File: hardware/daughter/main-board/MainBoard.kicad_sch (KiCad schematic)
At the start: 15 parts, among them J1 Conn_01x03_Pin, J2 Conn_01x03_Pin, J3 Conn_01x03_Pin, J4 Conn_01x03_Pin, SW1 SW_SP3T, SW2 SW_SP3T, U1 CD22M3494MQZ, U2 LM7321MAX/NOPB, U3 TL071, U4 TL071, U5 TL071, U6 TL071

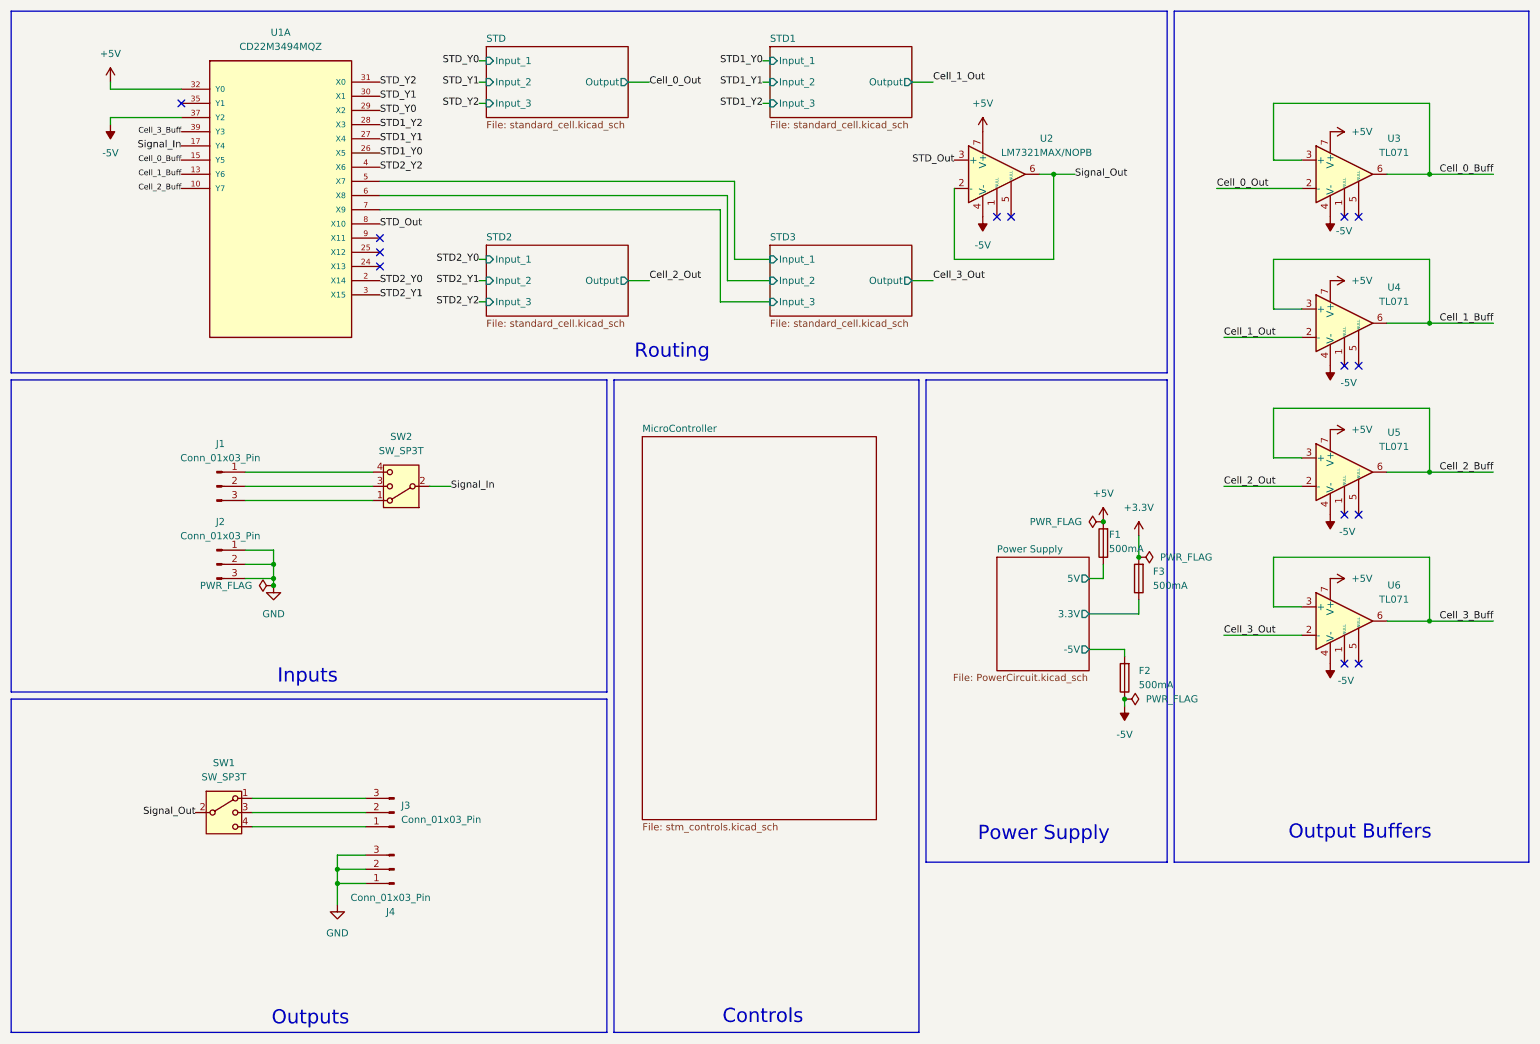
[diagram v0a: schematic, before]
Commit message: Updated daughter board schematic
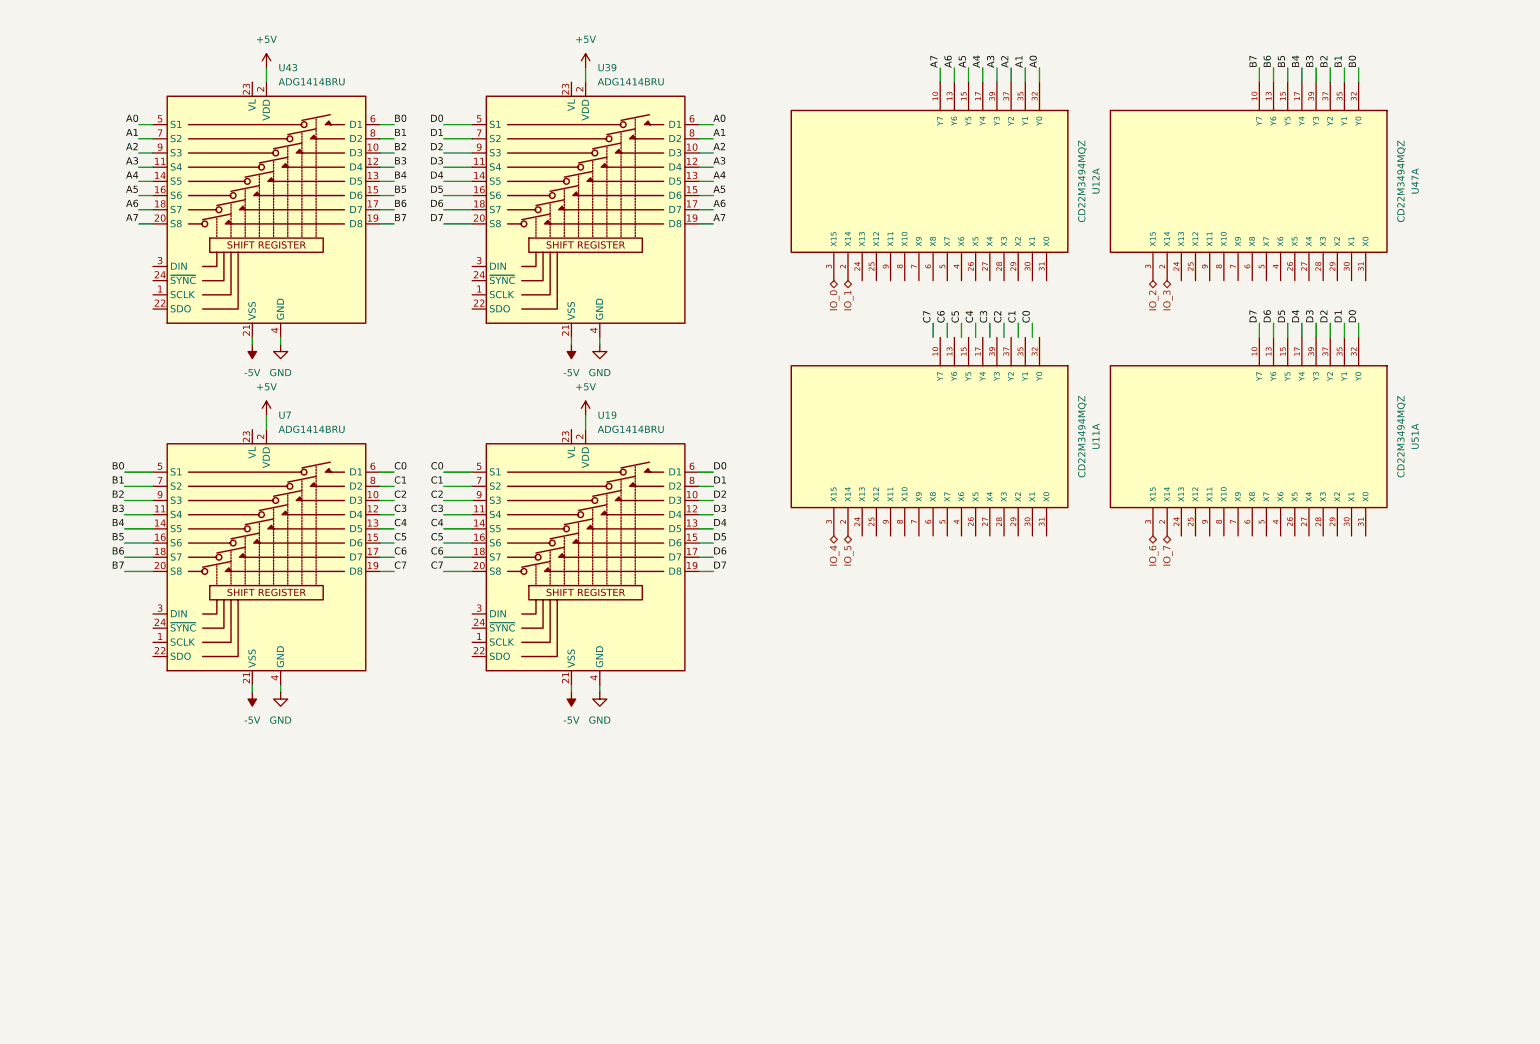
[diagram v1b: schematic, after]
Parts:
- removed F1, F2, F3: 500mA, Fuse:Fuse_0603_1608Metric_Pad1.05x0.95mm_HandSolder, symbol Device:Fuse
- removed J1, J2, J3, J4: Conn_01x03_Pin, Connector_PinHeader_2.54mm:PinHeader_1x03_P2.54mm_Vertical, symbol Connector:Conn_01x03_Pin
- removed SW1, SW2: SW_SP3T, Button_Switch_THT:SW_Slide_SP3T_Straight_CK_OS103012MU1QP1, symbol SeniorDesign:SW_SP3T_2P
- removed U1: CD22M3494MQZ, SeniorDesignFP:PLCC44_16P66X16P66_INR-M, symbol SeniorDesign:CD22M3494MQZ
- removed U2: LM7321MAX/NOPB, Package_SO:SOIC-8_3.9x4.9mm_P1.27mm, symbol Amplifier_Operational:TL081
- removed U3, U4, U5, U6: TL071, Package_SO:SOIC-8_3.9x4.9mm_P1.27mm, symbol Amplifier_Operational:TL071
- added U11, U12, U47, U51: CD22M3494MQZ, SeniorDesignFP:PLCC44_16P66X16P66_INR-M, symbol SeniorDesign:CD22M3494MQZ
- added U19, U39, U43, U7: ADG1414BRU, Package_SO:TSSOP-24_4.4x7.8mm_P0.65mm, symbol Analog_Switch:ADG1414BRU
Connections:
- net +5V: now also U19.2 (VDD), U39.2 (VDD), U43.2 (VDD), U7.2 (VDD)
- net -5V: now also U19.21 (VSS), U39.21 (VSS), U43.21 (VSS), U7.21 (VSS)
- net GND: now also U19.4 (GND), U39.4 (GND), U43.4 (GND), U7.4 (GND)
- new net A0: U12.32 (Y0), U39.6 (D1), U43.5 (S1)
- new net A1: U12.35 (Y1), U39.8 (D2), U43.7 (S2)
- new net A2: U12.37 (Y2), U39.10 (D3), U43.9 (S3)
- new net A3: U12.39 (Y3), U39.12 (D4), U43.11 (S4)
- new net A4: U12.17 (Y4), U39.13 (D5), U43.14 (S5)
- new net A5: U12.15 (Y5), U39.15 (D6), U43.16 (S6)
- new net A6: U12.13 (Y6), U39.17 (D7), U43.18 (S7)
- new net A7: U12.10 (Y7), U39.19 (D8), U43.20 (S8)
- new net B0: U43.6 (D1), U47.32 (Y0), U7.5 (S1)
- new net B1: U43.8 (D2), U47.35 (Y1), U7.7 (S2)
- new net B2: U43.10 (D3), U47.37 (Y2), U7.9 (S3)
- new net B3: U43.12 (D4), U47.39 (Y3), U7.11 (S4)
- new net B4: U43.13 (D5), U47.17 (Y4), U7.14 (S5)
- new net B5: U43.15 (D6), U47.15 (Y5), U7.16 (S6)
- new net B6: U43.17 (D7), U47.13 (Y6), U7.18 (S7)
- new net B7: U43.19 (D8), U47.10 (Y7), U7.20 (S8)
- new net C0: U19.5 (S1), U7.6 (D1)
- new net C1: U19.7 (S2), U7.8 (D2)
- new net C2: U19.9 (S3), U7.10 (D3)
- new net C3: U19.11 (S4), U7.12 (D4)
- new net C4: U19.14 (S5), U7.13 (D5)
- new net C5: U19.16 (S6), U7.15 (D6)
- new net C6: U19.18 (S7), U7.17 (D7)
- new net C7: U19.20 (S8), U7.19 (D8)
- new net D0: U19.6 (D1), U39.5 (S1), U51.32 (Y0)
- new net D1: U19.8 (D2), U39.7 (S2), U51.35 (Y1)
- new net D2: U19.10 (D3), U39.9 (S3), U51.37 (Y2)
- new net D3: U19.12 (D4), U39.11 (S4), U51.39 (Y3)
- new net D4: U19.13 (D5), U39.14 (S5), U51.17 (Y4)
- new net D5: U19.15 (D6), U39.16 (S6), U51.15 (Y5)
- new net D6: U19.17 (D7), U39.18 (S7), U51.13 (Y6)
- new net D7: U19.19 (D8), U39.20 (S8), U51.10 (Y7)
- new net IO_0: U12.3 (X15)
- new net IO_1: U12.2 (X14)
- new net IO_2: U47.3 (X15)
- new net IO_3: U47.2 (X14)
- new net IO_4: U11.3 (X15)
- new net IO_5: U11.2 (X14)
- new net IO_6: U51.3 (X15)
- new net IO_7: U51.2 (X14)
- no-connect marks 14 -> 0
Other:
- removed sheet MicroController
- removed sheet Power Supply
- removed sheet STD
- removed sheet STD1
- removed sheet STD2
- removed sheet STD3
- note removed: "Controls"
- note removed: "Inputs"
- note removed: "Output Buffers"
- note removed: "Outputs"
- note removed: "Power Supply"
- note removed: "Routing"
